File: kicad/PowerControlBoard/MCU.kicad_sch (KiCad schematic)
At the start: 8 parts, among them J11 LCD pinsocket, U2 ESP32-C5-DevKitC-1, U7 PCA9306

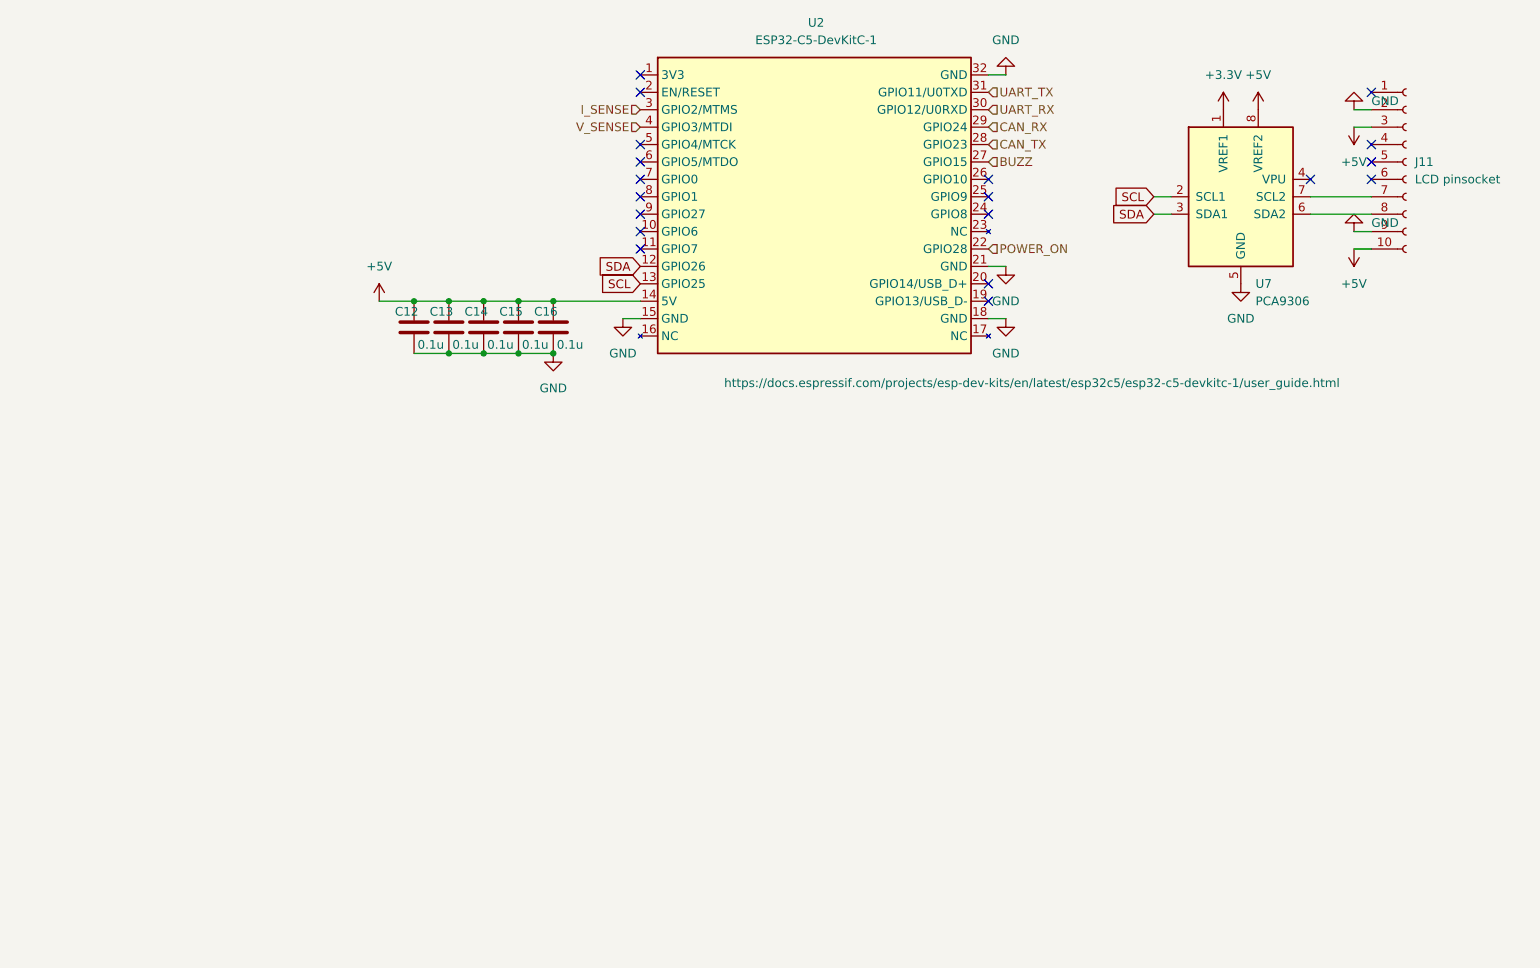
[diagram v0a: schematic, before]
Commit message: commit
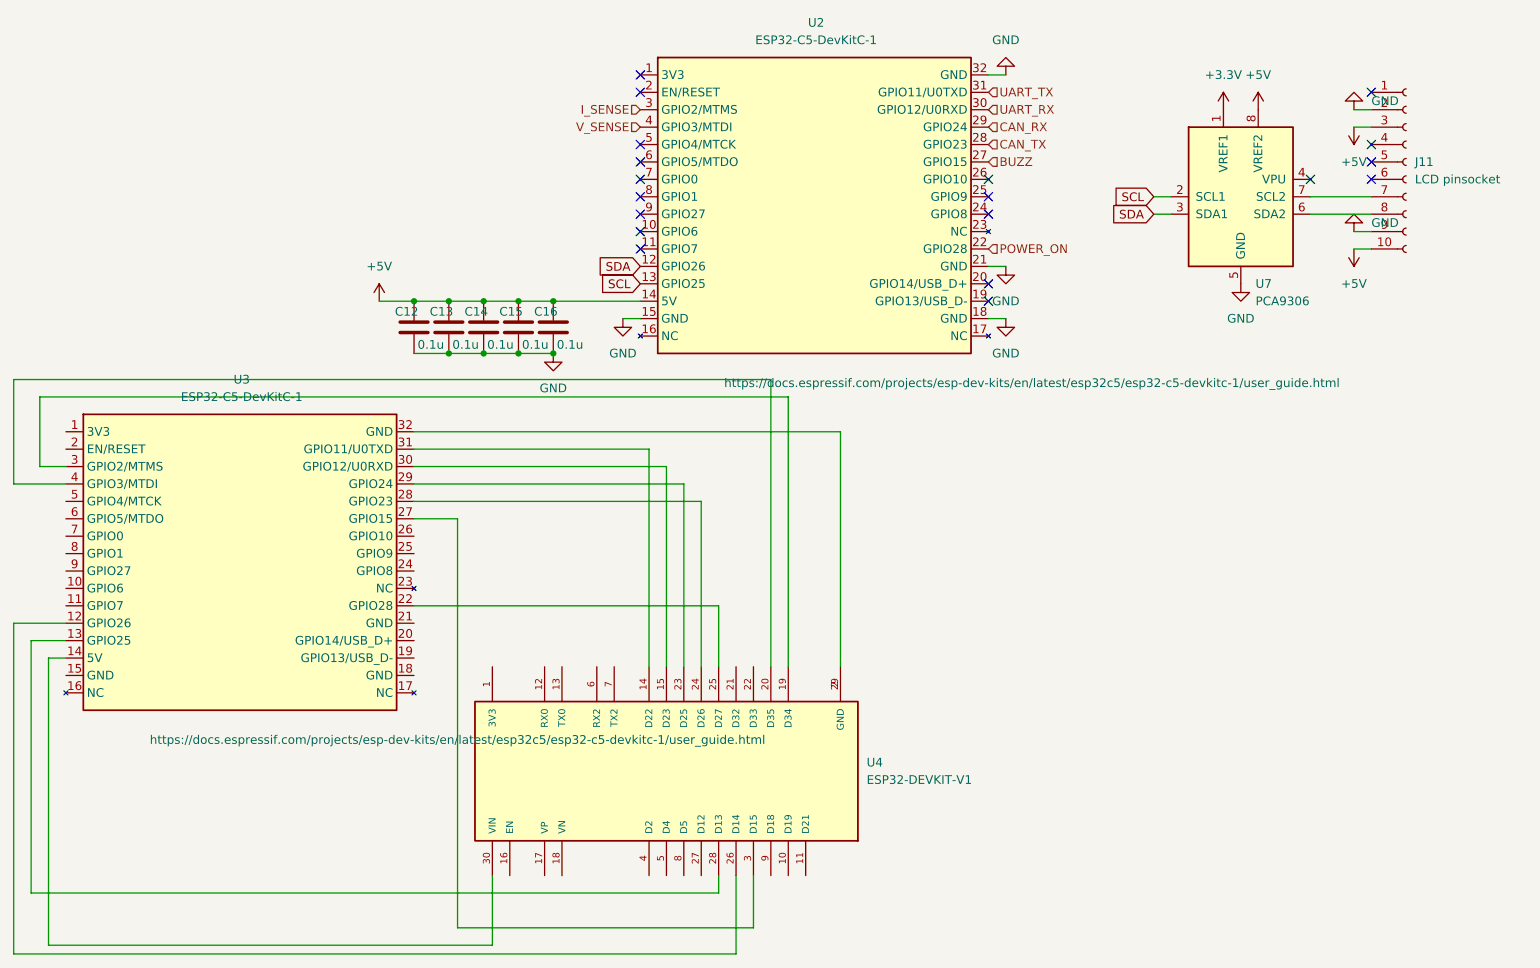
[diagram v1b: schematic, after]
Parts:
- added U3: ESP32-C5-DevKitC-1, PCM_Espressif:ESP32-C5-DevKitC-1, symbol Espressif:ESP32-C5-DevKitC-1
- added U4: ESP32-DEVKIT-V1, ESP32-DEVKIT-V1:MODULE_ESP32_DEVKIT_V1, symbol ESP32-DEVKIT-V1:ESP32-DEVKIT-V1
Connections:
- new net: U3.31 (GPIO11/U0TXD), U4.14 (D22)
- new net: U3.30 (GPIO12/U0RXD), U4.15 (D23)
- new net: U3.3 (GPIO2/MTMS), U4.19 (D34)
- new net: U3.32 (GND), U4.2 (GND), U4.29 (GND)
- new net: U3.4 (GPIO3/MTDI), U4.20 (D35)
- new net: U3.29 (GPIO24), U4.23 (D25)
- new net: U3.28 (GPIO23), U4.24 (D26)
- new net: U3.22 (GPIO28), U4.25 (D27)
- new net: U3.12 (GPIO26), U4.26 (D14)
- new net: U3.13 (GPIO25), U4.28 (D13)
- new net: U3.27 (GPIO15), U4.3 (D15)
- new net: U3.14 (5V), U4.30 (VIN)
